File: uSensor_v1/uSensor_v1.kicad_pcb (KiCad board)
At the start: 2 copper layers, 171 x 76.4 mm, 287 parts, among them J1 +12V Supply, J2 Conn_01x03, J3 Conn_01x03, J4 NS25-W8P 6-pin 2,54mm, J5 USB_B, J6 GNDA-GNDD Jumper, J7 Barrel_Jack_Switch, Q1 BC817-25, Q2 BC817-25, Q3 BC847PN-7-F, Q4 BC847PN-7-F, SW1 SW_Push, SW2 SW_Push, SW3 SW_Push, U1 AM10TW-2405DZ, U10 KSS-213 Connector, U11 AD7795, U12 AD5667, U13 TBD, U14 TBD, U15 REF192, U16 TBD, U17 TBD, U2 LD1117A, U22 RCLAMP, U3 STM32F407VGTx, U4 MCP9700AT, U5 MCP9700AT, U6 LM6132A, U7 MCP9700AT, U8 MCP9700AT, U9 UG-2864KSWLG01

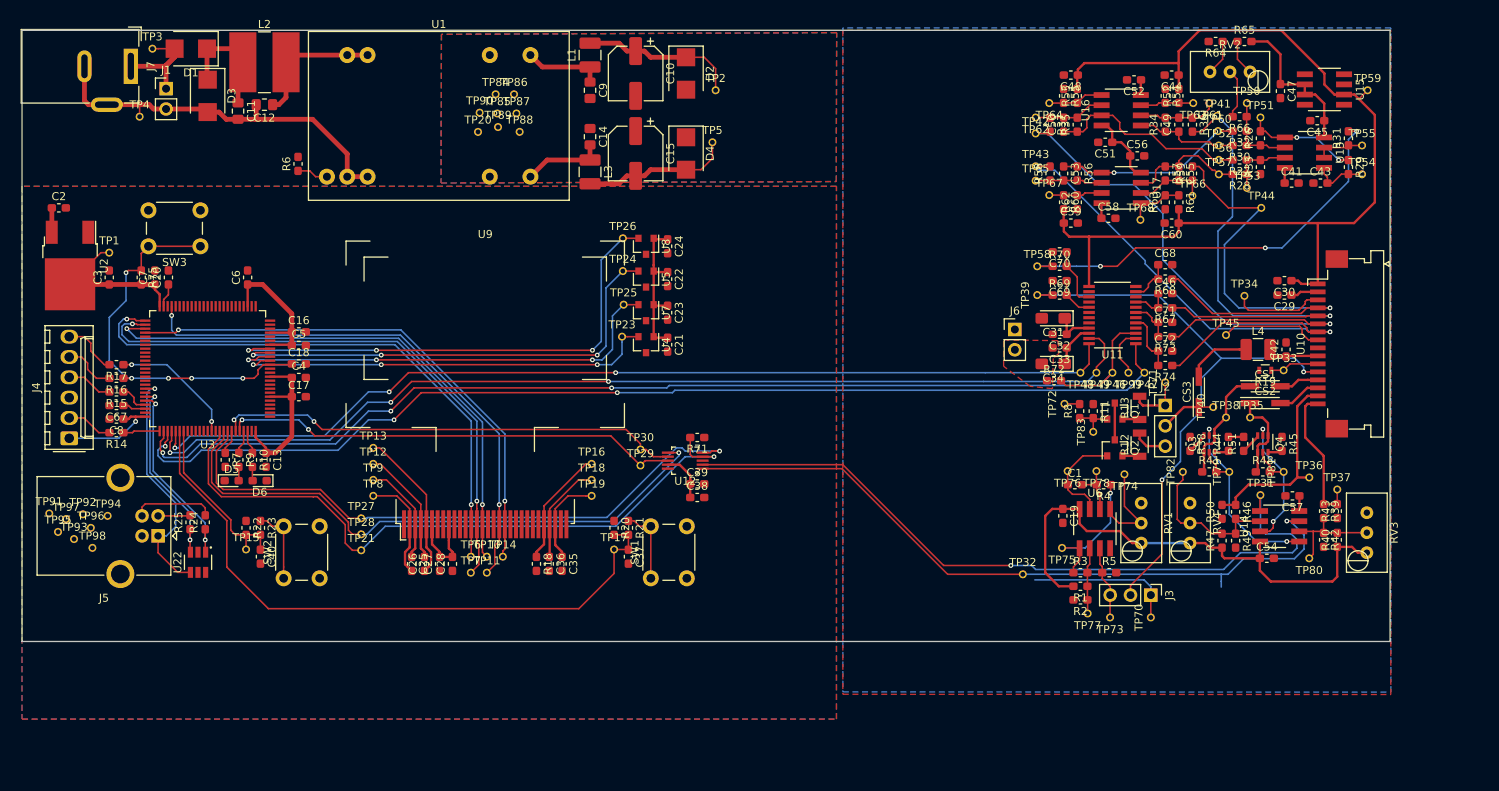
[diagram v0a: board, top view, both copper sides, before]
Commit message: Layout in progress.
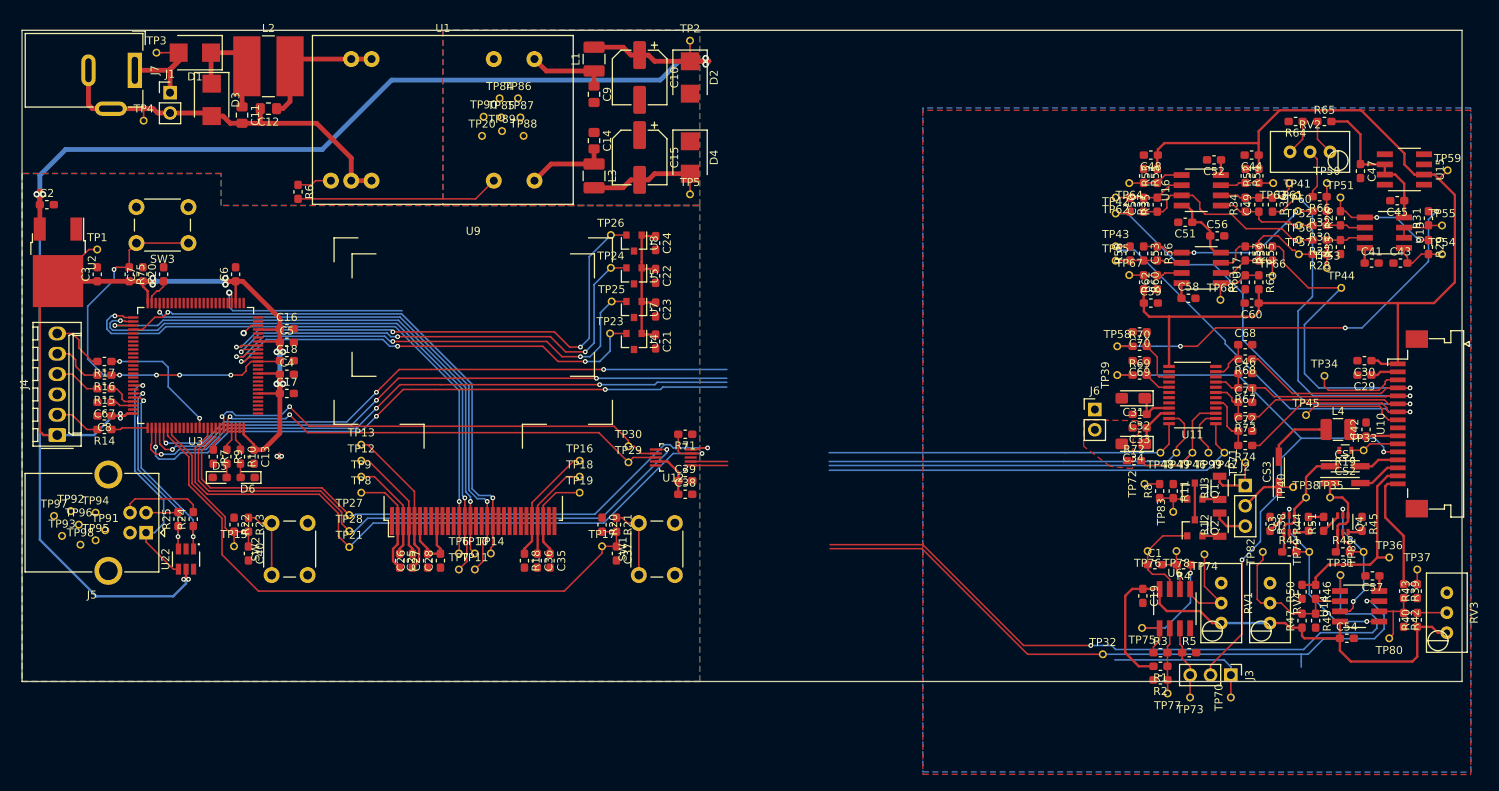
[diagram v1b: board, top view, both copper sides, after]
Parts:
- moved C56 14.1 mm to (162.4, 38.7)
- moved J2 14.1 mm to (165.9, 69.9)
- moved R27 14.1 mm to (175.2, 39.2)
- moved R74 14.1 mm to (165.9, 64.9)
- moved TP35 14.1 mm to (176.5, 71.4)
- moved TP38 14.1 mm to (173.5, 71.4)
- moved TP41 14.1 mm to (172.4, 33.7)
- moved TP56 14.1 mm to (172.6, 39.2)
- moved C1 14.1 mm to (154.6, 79.8)
- moved C19 14.1 mm to (153.1, 83.7)
- moved C29 14.1 mm to (180.8, 56.1)
- moved C30 14.1 mm to (180.8, 54.3)
- moved C31 14.1 mm to (151.9, 59.0)
- moved C32 14.1 mm to (152.7, 61.0)
- moved C33 14.1 mm to (152.7, 62.7)
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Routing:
- net +5V: track 129.5 -> 299.2 mm, vias 0 -> 6
- net +3V3: track 113.9 -> 171.8 mm, vias 1 -> 12
- net GNDA: track 0.00 -> 25.4 mm
- net DAC_LD_CTRL: track 1.91 -> 26.9 mm, vias 0 -> 1
- net LCD_SI: track 65.9 -> 70.1 mm
- net SWITCH_1: track 80.3 -> 76.3 mm
- net -5V: track 28.1 -> 24.8 mm
- net ADC_SCLK: track 136.1 -> 133.2 mm
- net LCD_A0: track 68.6 -> 71.1 mm
- net LCD_CS: track 70.6 -> 73.0 mm
- net LCD_RST: track 72.4 -> 74.8 mm
- net TEMP_SENS_OUT_1: track 53.2 -> 55.5 mm
- net SENS_PD_ADC: track 18.7 -> 20.9 mm, vias 0 -> 1
- net TEMP_SENS_OUT_2: track 56.9 -> 59.0 mm
- net ADC_DOUT: track 128.9 -> 127.0 mm
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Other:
- board size 171 x 76.4 mm -> 180 x 81.4 mm
